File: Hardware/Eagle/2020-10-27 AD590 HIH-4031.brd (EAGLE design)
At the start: 33 x 14 mm, 5 parts, among them IC1 AD590, U1 HIH-4031

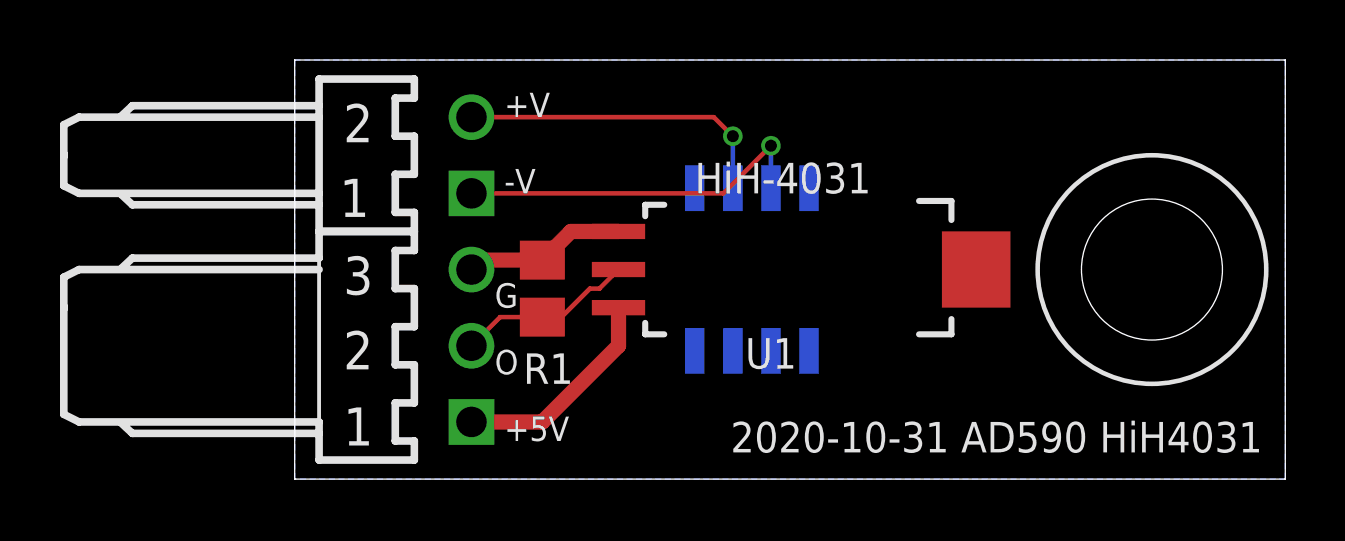
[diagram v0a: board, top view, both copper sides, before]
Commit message: Save minor changes
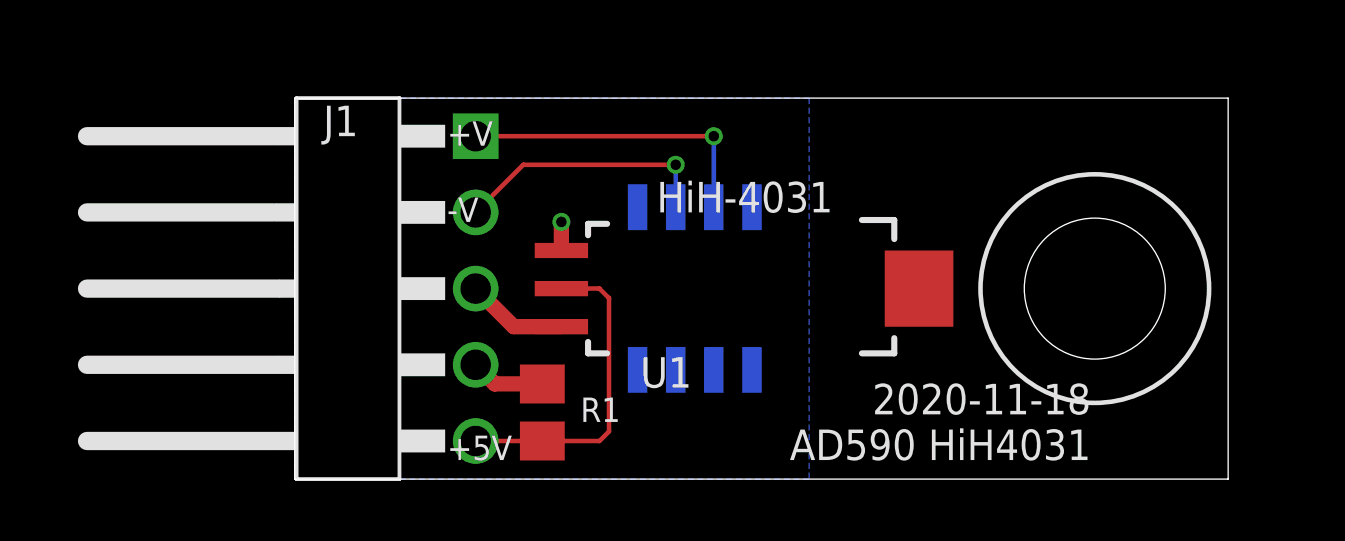
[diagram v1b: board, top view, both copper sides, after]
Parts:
- removed JP1: MOLEX 0022057028, AUmlib:MOLEX-7395-02-90DEG
- removed JP2: MOLEX 0022053031, AUmlib:MOLEX-7395-03-90DEG
- added J1: Molex 22122054, AUmlib:1X05RA-MOLEX-22122054
- moved R1 4.13 mm to (8.26, 2.22)
- moved IC1 2.01 mm to (13.3, 6.35)
- moved U1 2.01 mm to (14.0, 6.35)
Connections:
- net GND: now also J1.4; no longer JP2.3
- net OUT: now also J1.5; no longer JP2.2
- net V+: now also J1.2; no longer JP1.2
- net V-: now also J1.1; no longer JP1.1
- net VCC: now also J1.3; no longer JP2.1
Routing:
- net OUT: track 5.95 -> 10.7 mm
- net VCC: track 7.22 -> 3.38 mm
- net GND: track 5.43 -> 3.44 mm, vias 0 -> 1
- net V+: track 10.7 -> 8.74 mm
- net V-: track 12.1 -> 10.3 mm
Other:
- board size 33 x 14 mm -> 31.1 x 12.7 mm
- board text added: "2020-11-18 AD590 HiH4031"
- board text removed: "2020-10-31 AD590 HiH4031"
- board text removed: "G"
- board text removed: "O"
